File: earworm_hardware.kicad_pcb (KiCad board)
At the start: 4 copper layers, 19.1 x 26.3 mm, 49 parts, among them J1 Conn_01x05, J2 Conn_01x02, T1 LPR6235-752SMRC, U1 nRF54L15-QFXX, U2 ADXL367BCCZ-RL7, U3 LTC3108EDE-TRPBF, X1 32.768 kHz, X2 32MHz

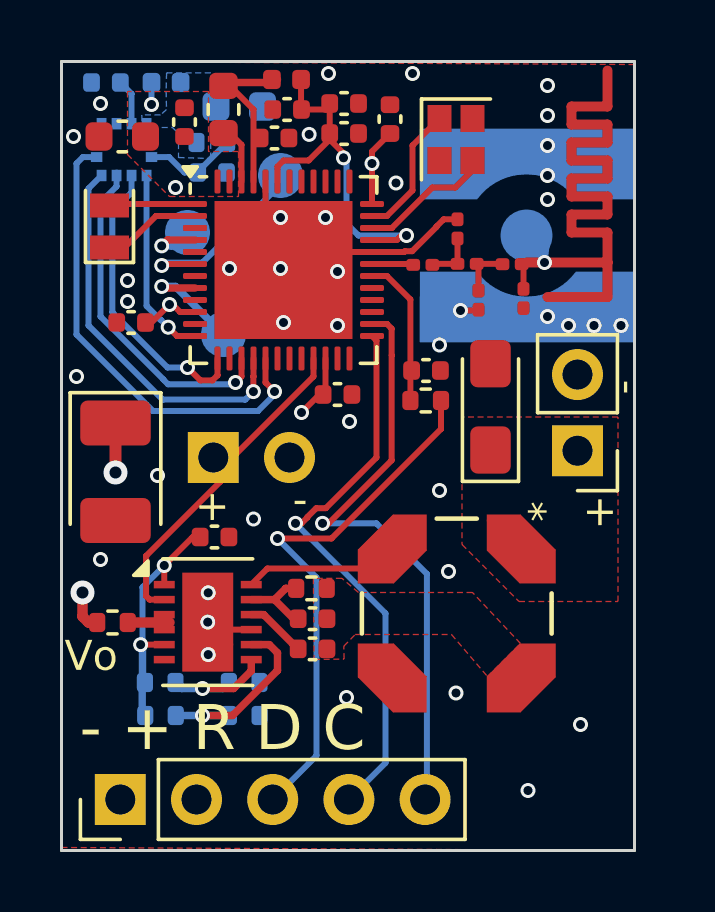
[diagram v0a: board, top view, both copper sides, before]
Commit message: various fixes
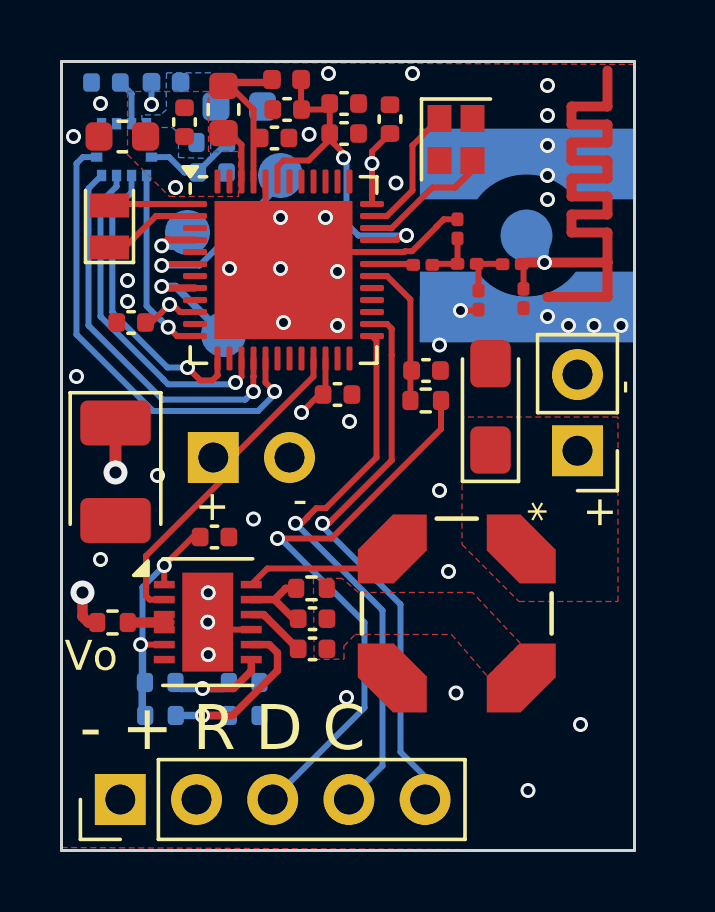
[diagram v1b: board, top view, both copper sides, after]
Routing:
- net /nRF54L15 RFSoC/NRST: track 17.7 -> 19.1 mm
- net /nRF54L15 RFSoC/SWCLK: track 19.3 -> 18.2 mm
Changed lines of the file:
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@@
 		)
 		(fp_text user "*"
-			(at -1.8415 0.75 -90)
-			(unlocked yes)
+			(at -1.8415 0.75 90)
 			(layer "B.SilkS")
 			(effects
@@
 		)
 		(fp_text user "*"
-			(at -1.8415 0.75 90)
+			(at -1.8415 0.75 -90)
+			(unlocked yes)
 			(layer "B.SilkS")
 			(effects
 				(font
-					(size 0.8 0.8)
+					(size 1 1)
 					(thickness 0.15)
 				)
@@
 		(fp_text user "*"
 			(at 0.1143 0.75 -90)
-			(unlocked yes)
 			(layer "B.Fab")
 			(effects
 				(font
-					(size 0.8 0.8)
+					(size 1 1)
 					(thickness 0.15)
 				)
@@
 		(pad "1" smd rect
 			(at -0.8636 0.750001)
-			(size 0.3302 0.381)
+			(size 0.3102 0.381)
 			(layers "B.Cu" "B.Paste" "B.Mask")
 			(net 40 "Net-(U1-P2.01)")
@@
 		(pad "2" smd rect
 			(at -0.8636 0.25)
-			(size 0.3302 0.381)
+			(size 0.3102 0.381)
 			(layers "B.Cu" "B.Paste" "B.Mask")
 			(net 51 "Net-(U1-P2.02)")
@@
 		(pad "3" smd rect
 			(at -0.8636 -0.25)
-			(size 0.3302 0.381)
+			(size 0.3102 0.381)
 			(layers "B.Cu" "B.Paste" "B.Mask")
 			(net 47 "Net-(U1-P2.04)")
@@
 		(pad "4" smd rect
 			(at -0.8636 -0.750001)
-			(size 0.3302 0.381)
+			(size 0.3102 0.381)
 			(layers "B.Cu" "B.Paste" "B.Mask")
 			(net 37 "Net-(U1-P2.05)")
@@
 		(pad "5" smd rect
 			(at -0.25 -0.9144 90)
-			(size 0.3302 0.381)
+			(size 0.31 0.381)
 			(layers "B.Cu" "B.Paste" "B.Mask")
 			(net 35 "Net-(U1-P2.06)")
@@
 		(pad "6" smd rect
 			(at 0.25 -0.9144 90)
-			(size 0.3302 0.381)
+			(size 0.3102 0.381)
 			(layers "B.Cu" "B.Paste" "B.Mask")
 			(net 27 "unconnected-(U2-INT2-Pad6)")
@@
 		(pad "7" smd rect
 			(at 0.8636 -0.750001)
-			(size 0.3302 0.381)
+			(size 0.3102 0.381)
 			(layers "B.Cu" "B.Paste" "B.Mask")
 			(net 2 "GND")
@@
 		(pad "8" smd rect
 			(at 0.8636 -0.25)
-			(size 0.3302 0.381)
+			(size 0.3102 0.381)
 			(layers "B.Cu" "B.Paste" "B.Mask")
 			(net 2 "GND")
@@
 		(pad "9" smd rect
 			(at 0.8636 0.25)
-			(size 0.3302 0.381)
+			(size 0.3102 0.381)
 			(layers "B.Cu" "B.Paste" "B.Mask")
 			(net 10 "Net-(U2-VREG_OUT)")
@@
 		(pad "10" smd rect
 			(at 0.8636 0.750001)
-			(size 0.3302 0.381)
+			(size 0.3102 0.381)
 			(layers "B.Cu" "B.Paste" "B.Mask")
 			(net 9 "Net-(U2-VS)")
@@
 		(pad "11" smd rect
 			(at 0.25 0.9144 90)
-			(size 0.3302 0.381)
+			(size 0.3102 0.381)
 			(layers "B.Cu" "B.Paste" "B.Mask")
 			(net 2 "GND")
@@
 		(pad "12" smd rect
 			(at -0.25 0.9144 90)
-			(size 0.3302 0.381)
+			(size 0.3102 0.381)
 			(layers "B.Cu" "B.Paste" "B.Mask")
 			(net 11 "Net-(U2-VDDIO)")
@@
 	)
 	(segment
-		(start 102.4 97.38)
-		(end 101.18 98.6)
+		(start 99.4 89.395)
+		(end 102.3 92.295)
 		(width 0.2)
 		(layer "B.Cu")
@@
 	)
 	(segment
-		(start 102.4 92.395)
-		(end 102.4 97.38)
+		(start 102.3 97.48)
+		(end 101.18 98.6)
 		(width 0.2)
 		(layer "B.Cu")
@@
 	)
 	(segment
-		(start 99.4 89.395)
-		(end 102.4 92.395)
+		(start 102.3 92.295)
+		(end 102.3 97.48)
 		(width 0.2)
 		(layer "B.Cu")
@@
 	)
 	(segment
-		(start 100.1 91.2)
-		(end 100.1 97.14)
+		(start 101.7 95.54)
+		(end 98.7 98.54)
 		(width 0.2)
 		(layer "B.Cu")
@@
 	)
 	(segment
-		(start 98.8 89.9)
-		(end 100.1 91.2)
+		(start 98.9 89.9)
+		(end 101.7 92.7)
 		(width 0.2)
 		(layer "B.Cu")
@@
 	)
 	(segment
-		(start 100.1 97.14)
-		(end 98.7 98.54)
+		(start 101.7 92.7)
+		(end 101.7 95.54)
+		(width 0.2)
+		(layer "B.Cu")
+		(net 19)
+	)
+	(segment
+		(start 98.8 89.9)
+		(end 98.9 89.9)
 		(width 0.2)
 		(layer "B.Cu")
@@
 	)
 	(segment
-		(start 103.78 91.08)
+		(start 102.9 97.02)
 		(end 103.78 97.9)
 		(width 0.2)
@@
 	)
 	(segment
-		(start 102.095 89.395)
-		(end 103.78 91.08)
+		(start 102.9 92.1)
+		(end 102.9 97.02)
+		(width 0.2)
+		(layer "B.Cu")
+		(net 20)
+	)
+	(segment
+		(start 100.300003 89.500003)
+		(end 102.9 92.1)
 		(width 0.2)
 		(layer "B.Cu")
@@
 	(segment
 		(start 100.300003 89.395)
-		(end 102.095 89.395)
+		(end 100.300003 89.500003)
 		(width 0.2)
 		(layer "B.Cu")
@@
 	)
 	(segment
-		(start 97.34 84.76)
-		(end 95.15 84.76)
+		(start 95 84.6)
+		(end 92.9 82.5)
 		(width 0.2)
 		(layer "B.Cu")
@@
 	)
 	(segment
-		(start 93.4356 78.1644)
-		(end 93.4356 77.7)
+		(start 97.34 84.76)
+		(end 95.15 84.76)
 		(width 0.2)
 		(layer "B.Cu")
@@
 	)
 	(segment
-		(start 92.9 78.7)
-		(end 93.4356 78.1644)
+		(start 95.15 84.76)
+		(end 94.99 84.6)
 		(width 0.2)
 		(layer "B.Cu")
@@
 	)
 	(segment
-		(start 95.15 84.76)
-		(end 94.99 84.6)
+		(start 92.9 78.7)
+		(end 93.4356 78.1644)
 		(width 0.2)
 		(layer "B.Cu")
@@
 	)
 	(segment
-		(start 95 84.6)
-		(end 92.9 82.5)
+		(start 97.4 84.7)
+		(end 97.34 84.76)
 		(width 0.2)
 		(layer "B.Cu")
@@
 	)
 	(segment
-		(start 97.4 84.7)
-		(end 97.34 84.76)
+		(start 93.4356 78.1644)
+		(end 93.4356 77.8)
 		(width 0.2)
 		(layer "B.Cu")
@@
 	)
 	(segment
-		(start 96.295 80.705)
-		(end 98.9 78.1)
-		(width 0.2)
-		(layer "B.Cu")
-		(net 59)
-	)
-	(segment
-		(start 95.035601 80.705)
-		(end 96.295 80.705)
+		(start 94.940601 80.8)
+		(end 96.2 80.8)
 		(width 0.2)
 		(layer "B.Cu")
@@
 	)
 	(segment
-		(start 94.940601 80.8)
-		(end 95.035601 80.705)
+		(start 96.2 80.8)
+		(end 98.9 78.1)
 		(width 0.2)
 		(layer "B.Cu")
